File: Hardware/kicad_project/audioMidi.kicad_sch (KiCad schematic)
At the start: 49 parts, among them J3 line_in, J4 headphone_out, J5 midi_in, J6 midi_out, U3 TLV320AIC3204, U4 AP3722AT_mic, U5 6N137, U7 apx804SR, U8 LM4890, U9 ME6211C

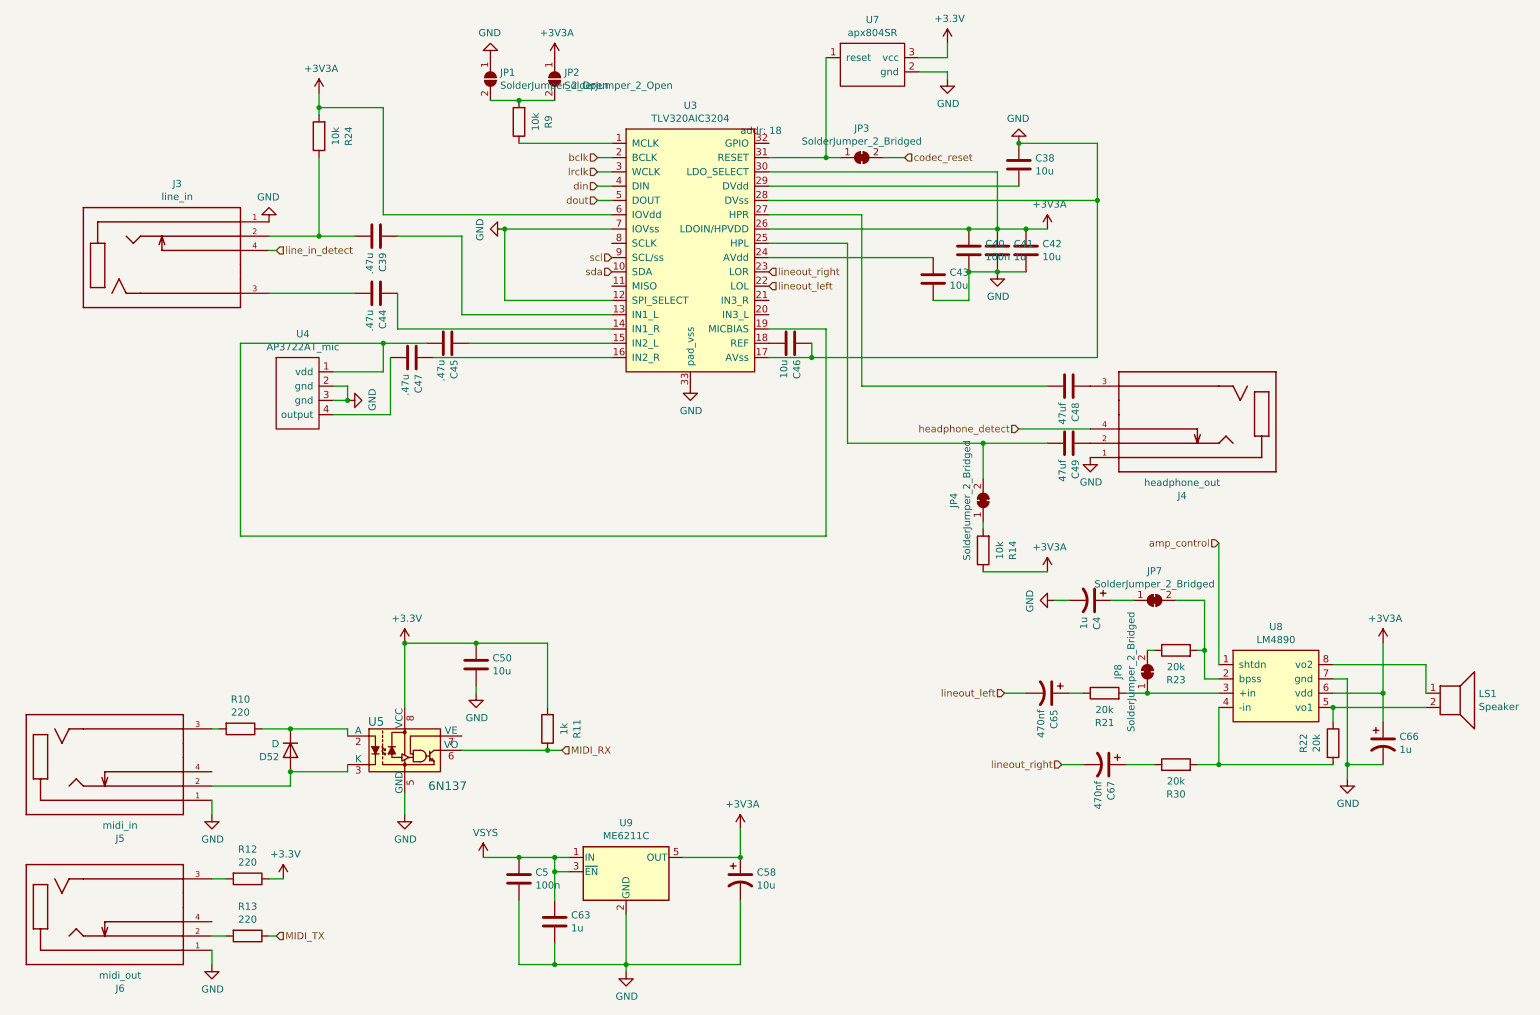
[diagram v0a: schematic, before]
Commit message: v9 hardware
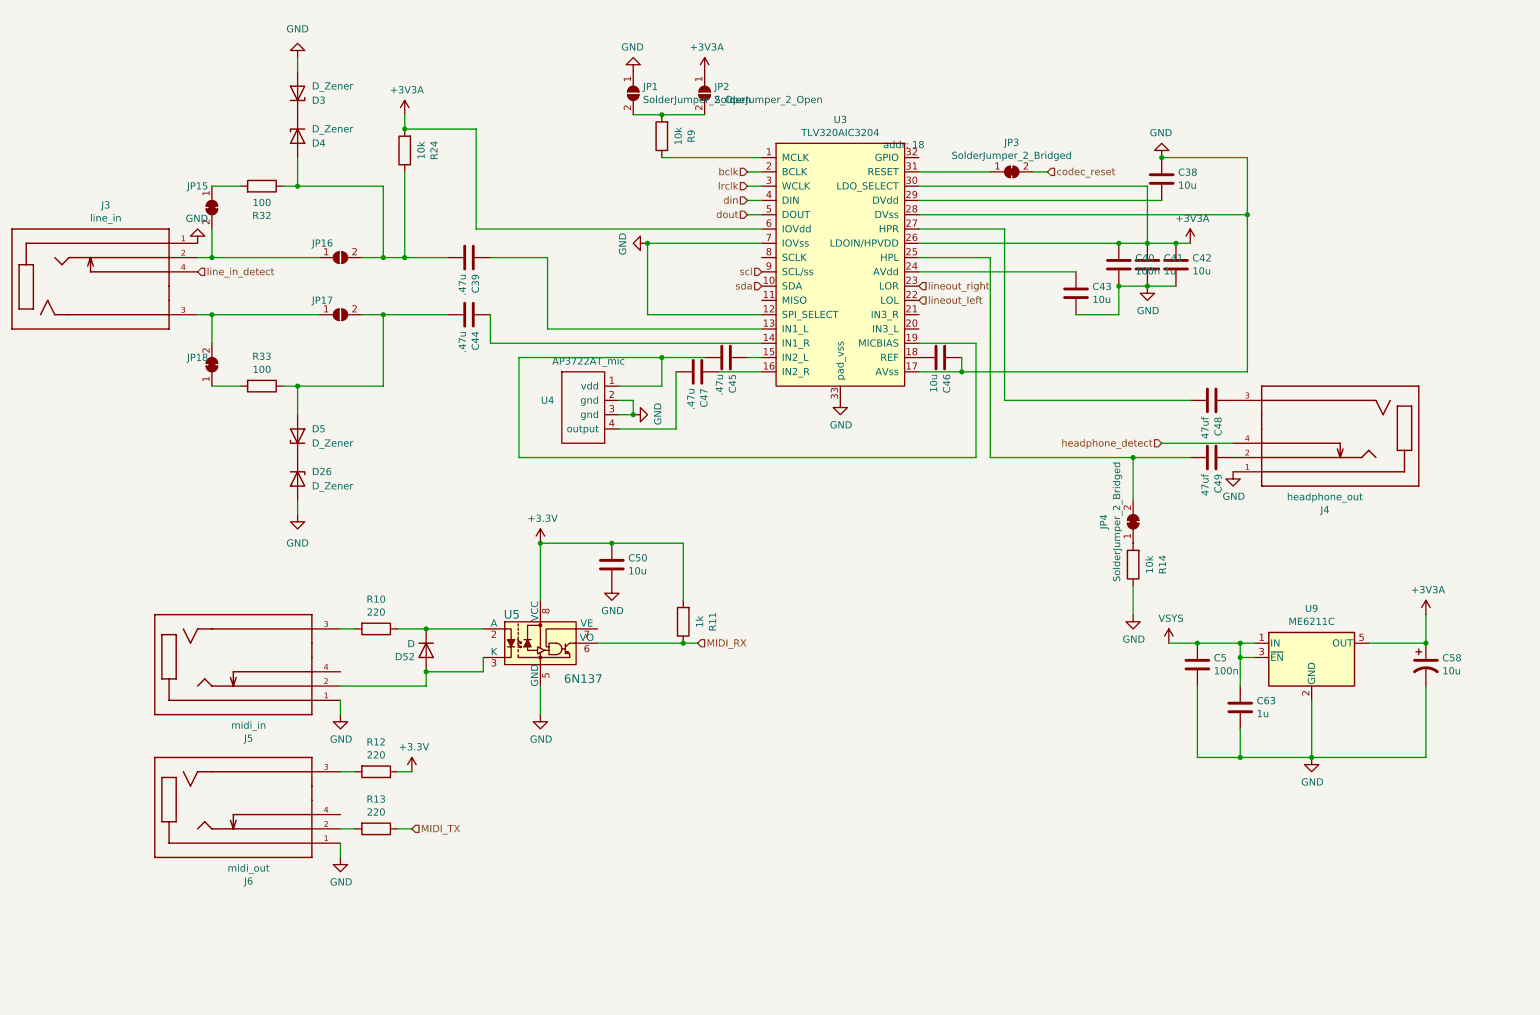
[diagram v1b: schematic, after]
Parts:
- removed C4, C66: 1u, Capacitors_Tantalum_SMD:CP_Tantalum_Case-A_EIA-3216-18_Reflow, symbol Device:CP1
- removed C65, C67: 470nf, Capacitors_Tantalum_SMD:CP_Tantalum_Case-A_EIA-3216-18_Reflow, symbol Device:CP1
- removed JP7, JP8: SolderJumper_2_Bridged, Jumper:SolderJumper-2_P1.3mm_Bridged_Pad1.0x1.5mm, symbol Jumper:SolderJumper_2_Bridged
- removed LS1: Speaker, Connector_PinHeader_2.54mm:PinHeader_1x02_P2.54mm_Horizontal, symbol Device:Speaker
- removed R21, R22, R23, R30: 20k, Resistors_SMD:R_0402_NoSilk, symbol Device:R
- removed U7: apx804SR, TO_SOT_Packages_SMD:SOT-23, symbol customLibrary:apx804SR
- removed U8: LM4890, Housings_SSOP:MSOP-8_3x3mm_Pitch0.65mm, symbol customLibrary:fm8002a
- added D26, D3, D4, D5: D_Zener, Diode_SMD:D_SOD-323F, symbol Device:D_Zener
- added JP15, JP18: SolderJumper_2_Bridged, Jumper:SolderJumper-2_P1.3mm_Bridged_Pad1.0x1.5mm, symbol Jumper:SolderJumper_2_Bridged
- added JP16, JP17: SolderJumper_2_Open, Jumper:SolderJumper-2_P1.3mm_Open_RoundedPad1.0x1.5mm, symbol Jumper:SolderJumper_2_Open
- added R32, R33: 100, Resistor_SMD:R_01005_0402Metric, symbol Device:R
- C39, C44, C45, C47: LCSC c1623 -> C1623
- C48, C49: LCSC C96123 -> C96123
- D52: LCSC c2128 -> C2128
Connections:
- net +3V3A: no longer R14.1
- net GND: now also R14.1, D26.2 (A), D3.2 (A)
- net at C39.2, R24.1: now also D4.2 (A), JP16.2 (B), R32.1; no longer J3.2 (TIP_1)
- net at C44.2: now also D5.2 (A), JP17.2 (B), R33.1; no longer J3.3 (RING)
- new net: J3.2 (TIP_1), JP15.2 (B), JP16.1 (A)
- new net: J3.3 (RING), JP17.1 (A), JP18.2 (B)
- new net: D3.1 (K), D4.1 (K)
- new net: JP15.1 (A), R32.2
- new net: JP18.1 (A), R33.2
- new net: D26.1 (K), D5.1 (K)
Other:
- moved on the sheet: C38, C39, C40, C41, C42, C43, C44, C45, C46, C47, C48, C49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
